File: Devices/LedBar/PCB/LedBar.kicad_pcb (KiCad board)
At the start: 2 copper layers, 63.5 x 99.3 mm, 167 parts, among them J1001 Conn_02x06_Odd_Even, J1002 Conn_02x06_Odd_Even, J1101 strip1_RGBW, J1102 Conn_01x05, J1103 Strip1_BRG, J1201 strip2_RGBW, J1202 Conn_02x06_Odd_Even, J1203 Strip3_RGBW, J1204 Strip2_BRG, J1205 Strip3_BRG, J1301 Conn_01x05, J1302 Strip4_RGBW, J1303 Strip4_BRG, J301 12VDC/5A, J401 RS485, J501 Left, J502 Center, J503 Right, J601 0-10V(1), J701 AVR-ISP-6, Q501 Si2302DS, Q502 Si2302DS, Q503 Si2302DS, Q504 Si2302DS, Q505 Si2302DS, Q506 Si2302DS, Q507 Si2302DS, Q508 Si2302DS, Q509 Si2302DS, Q510 Si2302DS, Q511 Si2302DS, Q512 Si2302DS, Q513 Si2302DS, Q514 Si2302DS, Q515 Si2302DS, Q516 Si2302DS, SW701 button, SW702 reset, SW703 SW_DIP_x05, U301 INA219AxD, U302 AMS1117-5.0, U401 ISO3082DW, U402 B0505S-1W-SIP4, U501 PCA9685PW, U601 LM393, U701 ATmega328P-AU, U901 DS1307Z+, Y701 14.7456Mhz, Y901 23.768kHz

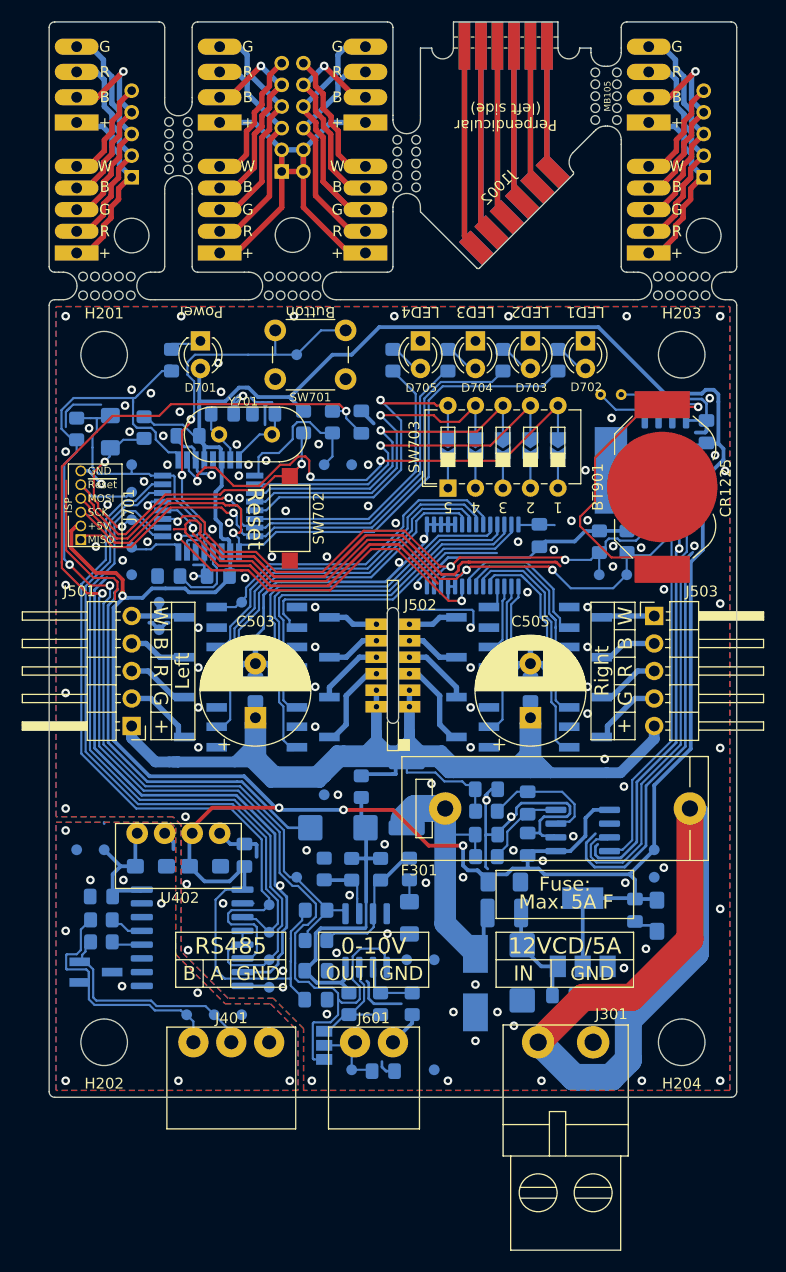
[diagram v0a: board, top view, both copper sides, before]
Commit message: Synchronized Mainboard pcbs
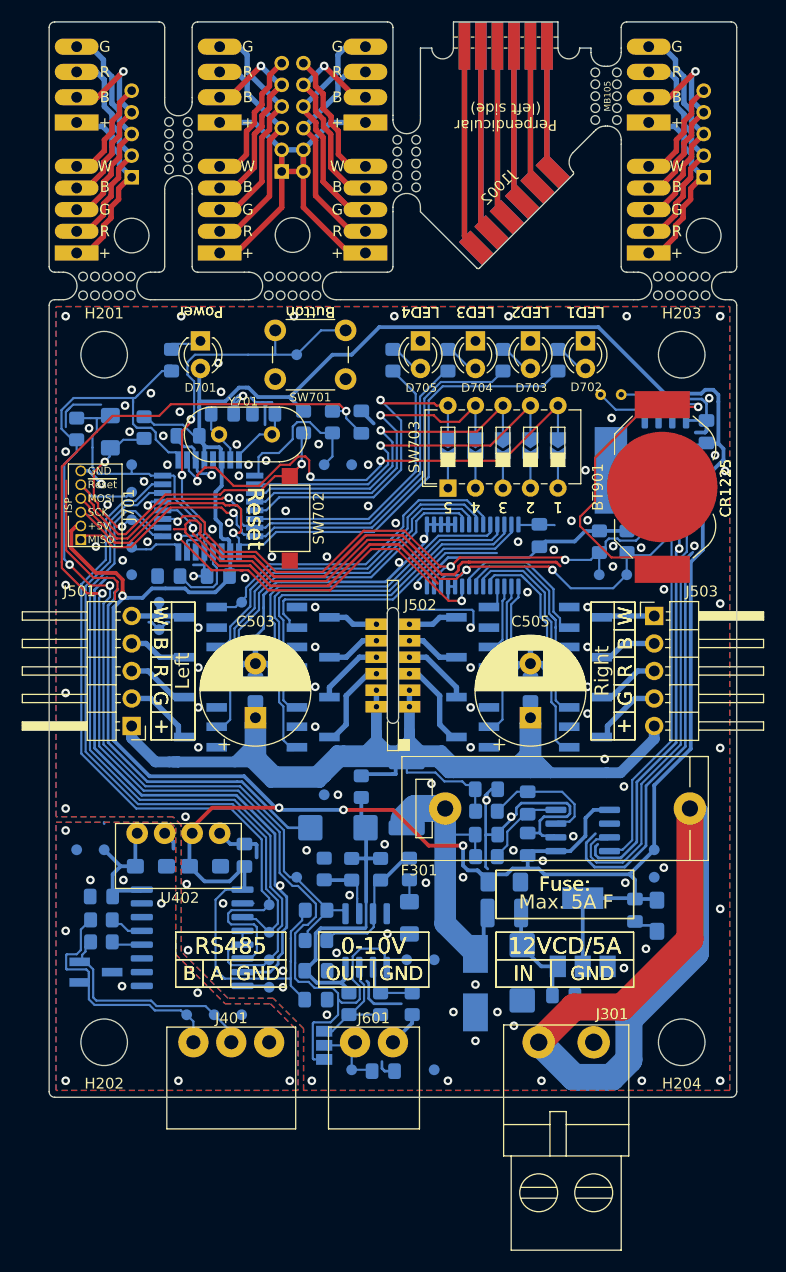
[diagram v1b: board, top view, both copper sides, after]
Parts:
- moved J301 0.05 mm to (169.7, 139.7)
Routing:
- net Net-(C601-Pad1): track 8.52 -> 9.26 mm
